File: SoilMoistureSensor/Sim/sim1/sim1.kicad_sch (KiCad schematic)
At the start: 38 parts, among them U1 74AUC1G86, U10 74AUC1G66, U11 74AUC1G66, U12 74AUC1G66, U13 TLV9001IDCK, U14 TLV9001IDCK, U2 74AUC1G86, U3 74AUC1G86, U4 74AUC1G86, U5 74AUC1G08, U6 74AUC1G08, U7 OPA356xxDBV, U8 OPA356xxDBV, U9 74AUC1G66

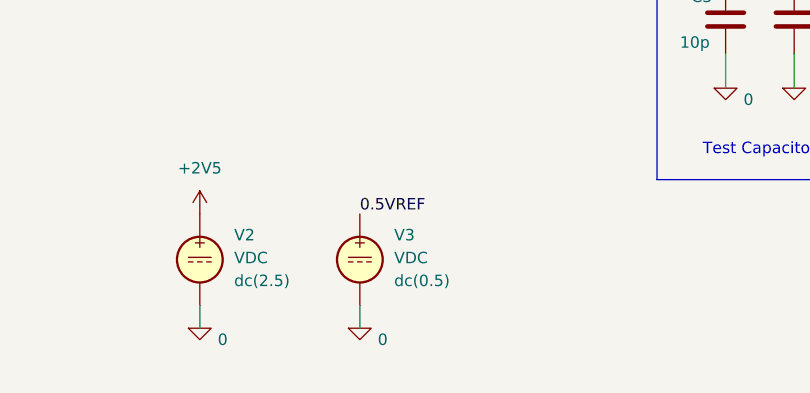
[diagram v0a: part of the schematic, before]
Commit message: wip
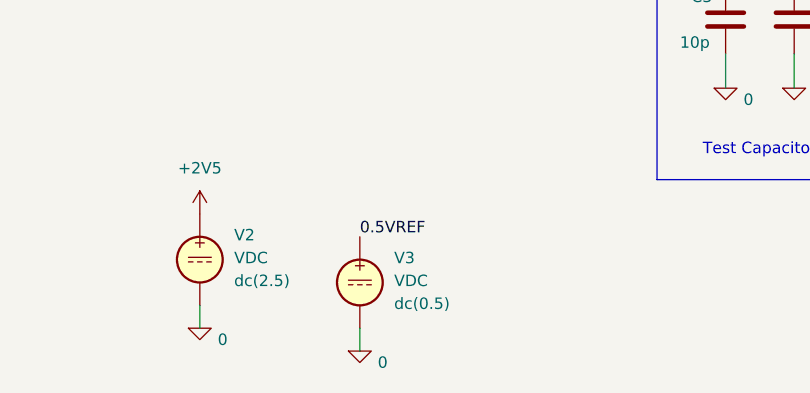
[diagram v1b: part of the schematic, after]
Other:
- moved on the sheet: V3
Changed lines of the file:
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@@
     (stroke (width 0) (type default) (color 0 0 0 0))
   )
-  (wire (pts (xy 67.31 173.99) (xy 67.31 176.53))
+  (wire (pts (xy 67.31 176.53) (xy 67.31 179.07))
     (stroke (width 0) (type default) (color 0 0 0 0))
   )
@@
     (effects (font (size 1.27 1.27)) (justify left bottom))
   )
-  (label "0.5VREF" (at 67.31 163.83 0)
+  (label "0.5VREF" (at 67.31 166.37 0)
     (effects (font (size 1.27 1.27)) (justify left bottom))
   )
@@
     )
   )
-  (symbol (lib_id "pspice:0") (at 67.31 176.53 0) (unit 1)
-    (in_bom yes) (on_board yes)
-    (property "Reference" "#GND021" (id 0) (at 67.31 179.07 0)
-      (effects (font (size 1.27 1.27)) hide)
-    )
-    (property "Value" "0" (id 1) (at 69.85 177.8 0))
-    (property "Footprint" "" (id 2) (at 67.31 176.53 0)
-      (effects (font (size 1.27 1.27)) hide)
-    )
-    (property "Datasheet" "~" (id 3) (at 67.31 176.53 0)
+  (symbol (lib_id "pspice:0") (at 67.31 179.07 0) (unit 1)
+    (in_bom yes) (on_board yes)
+    (property "Reference" "#GND021" (id 0) (at 67.31 181.61 0)
+      (effects (font (size 1.27 1.27)) hide)
+    )
+    (property "Value" "0" (id 1) (at 69.85 180.34 0))
+    (property "Footprint" "" (id 2) (at 67.31 179.07 0)
+      (effects (font (size 1.27 1.27)) hide)
+    )
+    (property "Datasheet" "~" (id 3) (at 67.31 179.07 0)
       (effects (font (size 1.27 1.27)) hide)
     )
@@
     (pin "1")
   )
-  (symbol (lib_id "Simulation_SPICE:VDC") (at 67.31 168.91 0) (unit 1)
+  (symbol (lib_id "Simulation_SPICE:VDC") (at 67.31 171.45 0) (unit 1)
     (in_bom yes) (on_board yes) (fields_autoplaced)
-    (property "Reference" "V3" (id 0) (at 71.12 166.1801 0)
+    (property "Reference" "V3" (id 0) (at 71.12 168.7201 0)
       (effects (font (size 1.27 1.27)) (justify left))
     )
-    (property "Value" "VDC" (id 1) (at 71.12 168.7201 0)
+    (property "Value" "VDC" (id 1) (at 71.12 171.2601 0)
       (effects (font (size 1.27 1.27)) (justify left))
     )
-    (property "Footprint" "" (id 2) (at 67.31 168.91 0)
-      (effects (font (size 1.27 1.27)) hide)
-    )
-    (property "Datasheet" "~" (id 3) (at 67.31 168.91 0)
-      (effects (font (size 1.27 1.27)) hide)
-    )
-    (property "Spice_Netlist_Enabled" "Y" (id 4) (at 67.31 168.91 0)
+    (property "Footprint" "" (id 2) (at 67.31 171.45 0)
+      (effects (font (size 1.27 1.27)) hide)
+    )
+    (property "Datasheet" "~" (id 3) (at 67.31 171.45 0)
+      (effects (font (size 1.27 1.27)) hide)
+    )
+    (property "Spice_Netlist_Enabled" "Y" (id 4) (at 67.31 171.45 0)
       (effects (font (size 1.27 1.27)) (justify left) hide)
     )
-    (property "Spice_Primitive" "V" (id 5) (at 67.31 168.91 0)
+    (property "Spice_Primitive" "V" (id 5) (at 67.31 171.45 0)
       (effects (font (size 1.27 1.27)) (justify left) hide)
     )
-    (property "Spice_Model" "dc(0.5)" (id 6) (at 71.12 171.2601 0)
+    (property "Spice_Model" "dc(0.5)" (id 6) (at 71.12 173.8001 0)
       (effects (font (size 1.27 1.27)) (justify left))
     )
